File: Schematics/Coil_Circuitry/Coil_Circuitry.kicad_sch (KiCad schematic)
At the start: 1 part, among them Q1 Q_NMOS_DGS

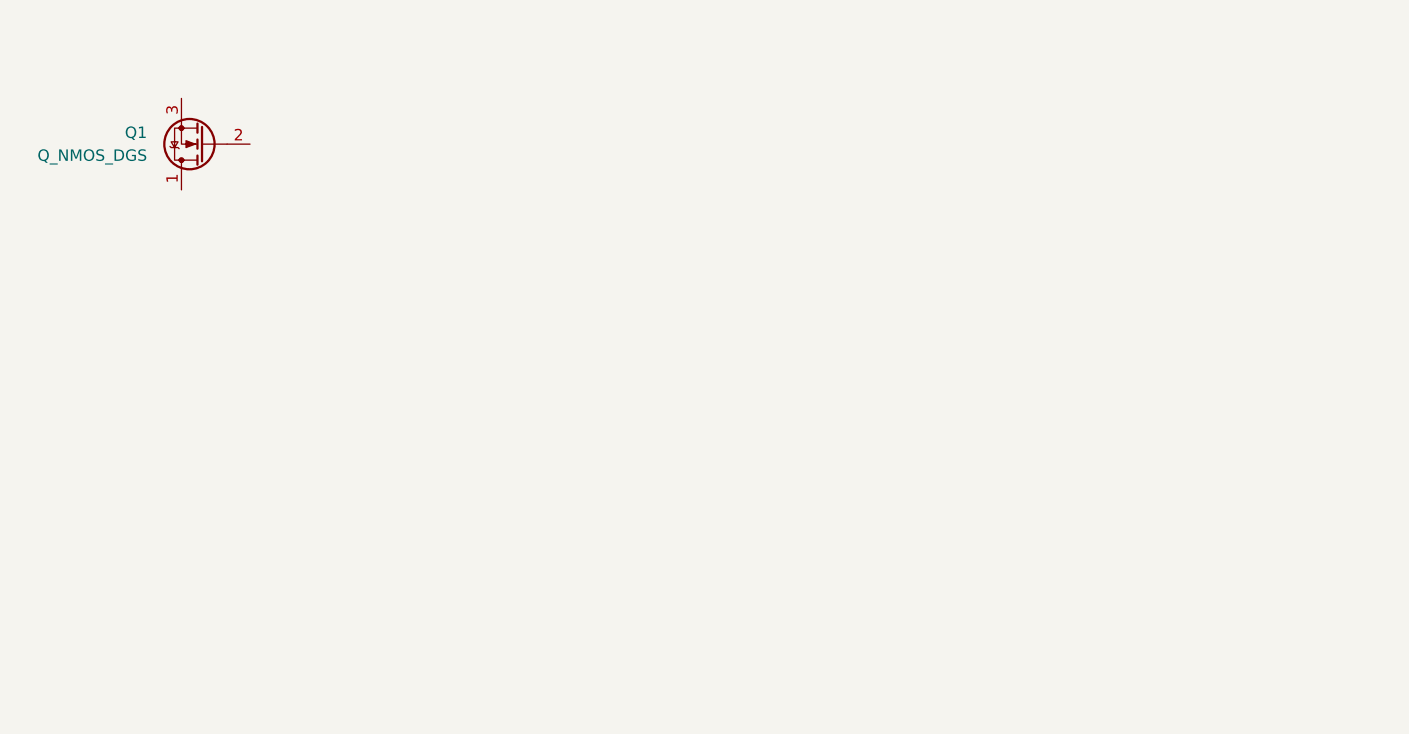
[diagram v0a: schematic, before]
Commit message: first draft circuit
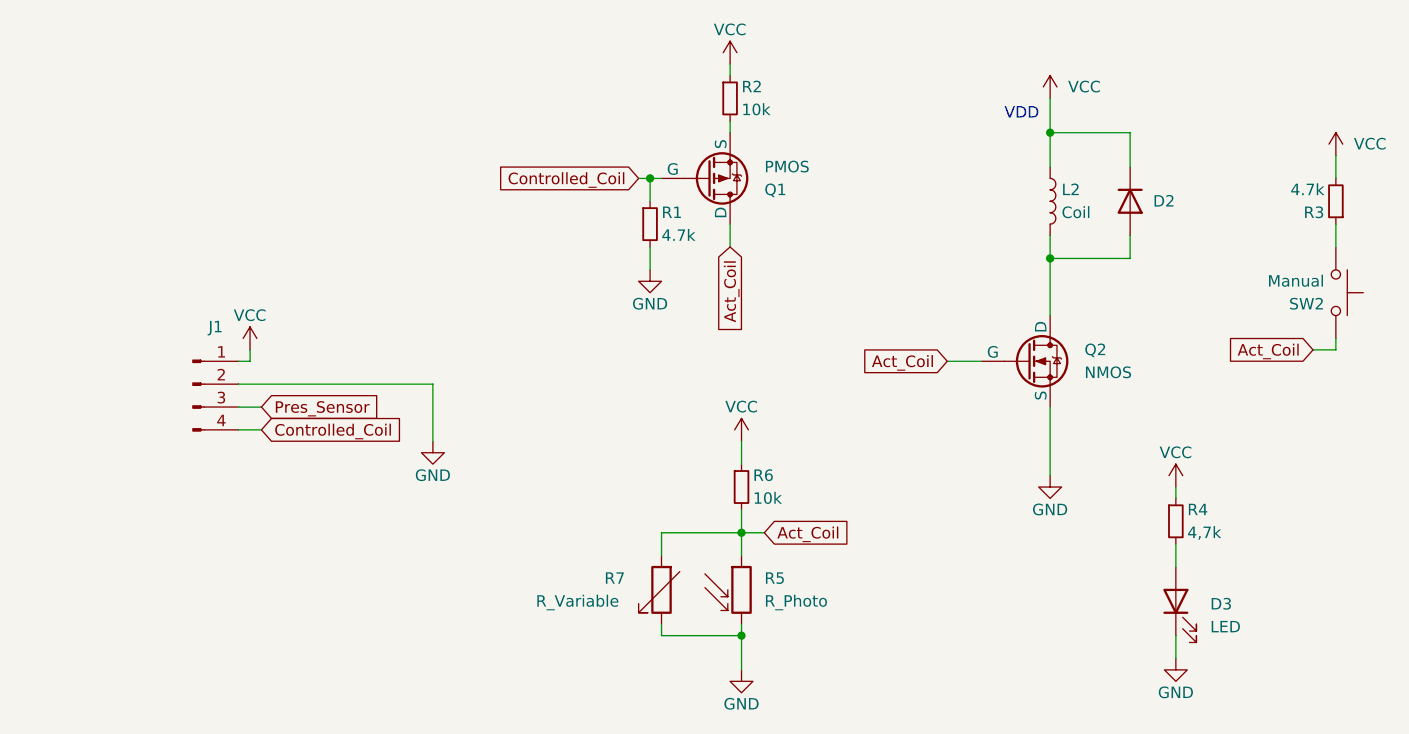
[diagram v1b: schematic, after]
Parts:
- removed Q1: Q_NMOS_DGS, symbol Device:Q_NMOS_DGS
- added D2: 1N914WT, Diode_SMD:D_SOD-523, symbol Diode:1N914WT
- added D3: LED, symbol Device:LED
- added J1: Conn_01x04_Pin, symbol Connector:Conn_01x04_Pin
- added L2: Coil, symbol Device:L
- added Q1: PMOS, symbol Simulation_SPICE:PMOS
- added Q2: NMOS, symbol Simulation_SPICE:NMOS
- added R1, R3: 4.7k, symbol Device:R_Small
- added R2, R6: 10k, symbol Device:R_Small
- added R4: 4,7k, symbol Device:R_Small
- added R5: R_Photo, symbol Device:R_Photo
- added R7: R_Variable, symbol Device:R_Variable
- added SW2: Manual, symbol Switch:SW_Push
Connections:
- new net: Q1.3 (S), R2.2
- new net: D3.2 (A), R4.2
- new net: R3.1, SW2.1
- new net: D2.2 (A), L2.2, Q2.1 (D)
- new net Act_Coil: Q1.1 (D), Q2.2 (G), R5.1, R6.2, R7.2, SW2.2
- new net Controlled_Coil: J1.4 (Pin_4), Q1.2 (G), R1.1
- new net GND: D3.1 (K), J1.2 (Pin_2), Q2.3 (S), R1.2, R5.2, R7.1
- new net Pres_Sensor: J1.3 (Pin_3)
- new net VCC: D2.1 (K), J1.1 (Pin_1), L2.1, R2.1, R3.2, R4.1, R6.1
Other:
- note added: "VDD"
